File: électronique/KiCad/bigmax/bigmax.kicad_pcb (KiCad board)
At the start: 2 copper layers, 99.1 x 99.1 mm, 25 parts, among them SW1 SW_Push, U1 qtr-1rc_a, U10 batt_connector, U11 micro_start, U2 qtr-1rc_b, U3 dc_geared_encoder, U4 dc_geared_encoder, U5 TPS61090_dc_boost, U6 MT3608, U7 VL53L0X_a, U8 VL53L0X_b, U9 dc_driver_1A_3-14V

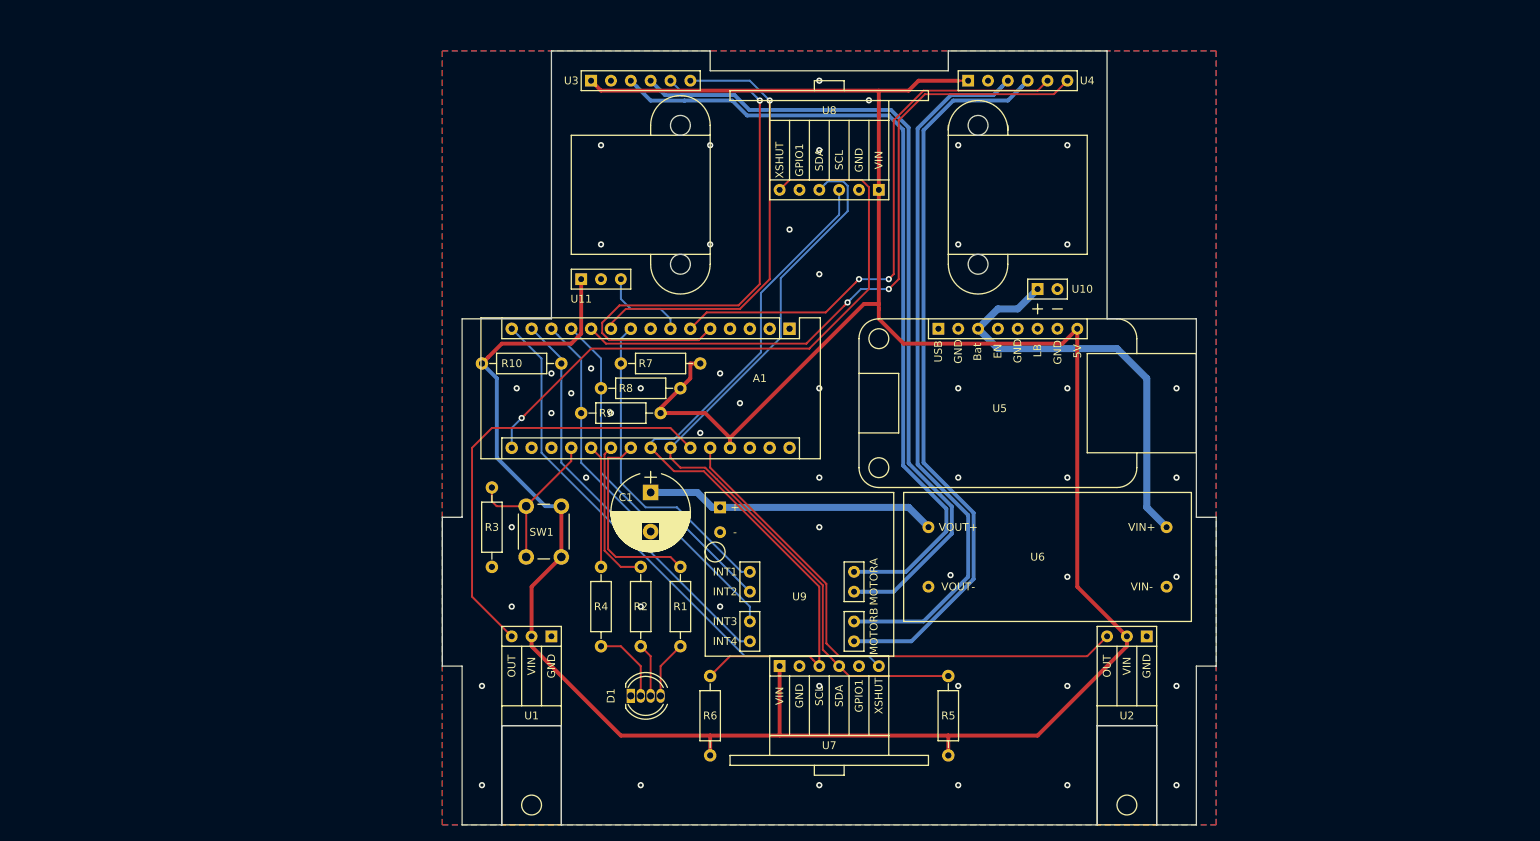
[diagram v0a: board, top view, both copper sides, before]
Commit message: Bigmax v2 - mai 2019
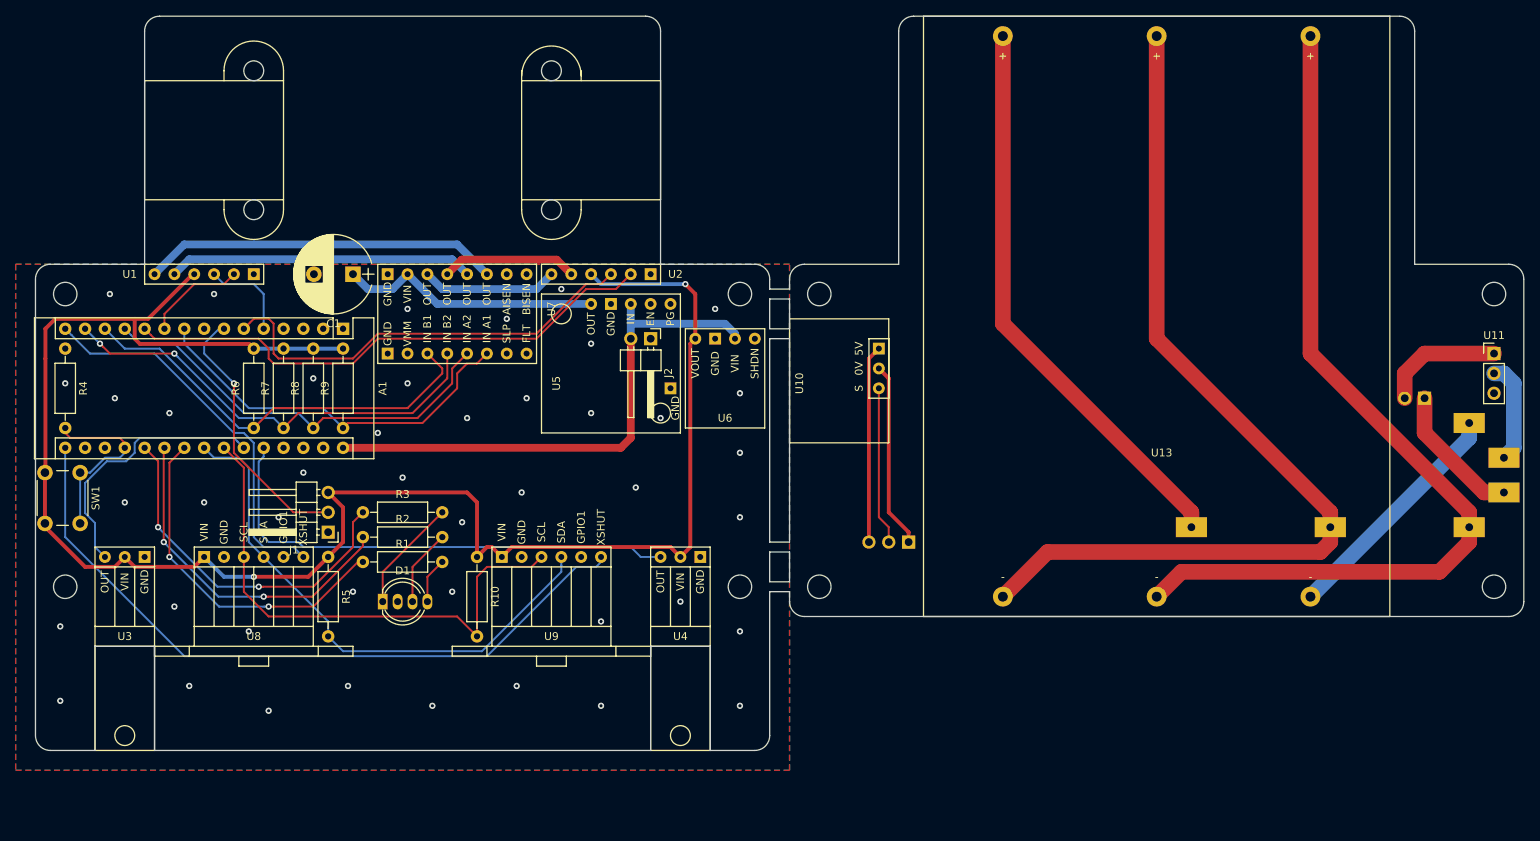
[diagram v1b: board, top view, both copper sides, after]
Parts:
- added J1: Conn_01x03, Pin_Headers:Pin_Header_Angled_1x03_Pitch2.54mm, F.Cu at (85.7, 112.4)
- added J2: Conn_01x02, Pin_Headers:Pin_Header_Angled_1x02_Pitch2.54mm, F.Cu at (127.0, 87.6)
- added J3: Conn_01x03_input, Pin_Headers:Pin_Header_Angled_1x03_Pitch2.54mm, B.Cu at (160.0, 113.7)
- added J4: Conn_01x02, Pin_Headers:Pin_Header_Angled_1x02_Pitch2.54mm, B.Cu at (226.1, 95.2)
- added U12: generic_bms_3s_10A, bigmax:generic_bms_3s_10A, B.Cu at (236.2, 102.9)
- added U13: generic_18650_3s_case, bigmax:CB-18650-PC6, F.Cu at (172.1, 48.9)
- D1: footprint LEDs:LED_D5.0mm-4 -> bigmax:LED_D5.0mm-4
- R3: value 1k -> 220
- R4: value 220 -> 1k
- U1: value qtr-1rc_a -> pololu_enc03b; footprint bigmax:qtr_1rc -> bigmax:pololu_enc03b
- U10: value batt_connector -> jsumo_micro_start; footprint bigmax:batt_connector -> bigmax:jsumo_micro_start
- U11: value micro_start -> generic_vertical_slide_switch; footprint bigmax:micro_start -> Pin_Headers:Pin_Header_Straight_1x03_Pitch2.54mm
- U2: value qtr-1rc_b -> pololu_enc03b; footprint bigmax:qtr_1rc -> bigmax:pololu_enc03b
- U3, U4: value dc_geared_encoder -> pololu_irs01a; footprint bigmax:dc_geared_encoder -> bigmax:pololu_irs01a
- U5: value TPS61090_dc_boost -> pololu_reg19a; footprint bigmax:dc_boost_500C -> bigmax:pololu_reg19a
- U6: value MT3608 -> pololu_reg04b; footprint bigmax:MT3608 -> bigmax:pololu_reg04b
- U7: value VL53L0X_a -> pololu_md17a; footprint bigmax:vl53l0x -> bigmax:pololu_md17a
- U8: value VL53L0X_b -> generic_vl53l0x; footprint bigmax:vl53l0x -> bigmax:generic_vl53l0x
- U9: value dc_driver_1A_3-14V -> generic_vl53l0x; footprint bigmax:MX1616 -> bigmax:generic_vl53l0x
- moved U11 117.2 mm to (234.9, 89.5)
- moved U8 98.3 mm to (69.8, 115.6), turned to 0 degrees
- moved U3 83.6 mm to (62.2, 115.6), turned to 180 degrees
- moved R5 80.8 mm to (85.7, 115.6)
- moved U2 78.6 mm to (127.0, 79.4)
- moved R4 74.1 mm to (52.1, 88.9)
- moved U4 69.9 mm to (133.3, 115.6), turned to 180 degrees
- moved R6 66.5 mm to (76.2, 99.1), turned to 90 degrees
- moved U7 64.2 mm to (93.3, 89.5), turned to 90 degrees
- moved U6 62.6 mm to (135.3, 87.6)
- moved SW1 61.7 mm to (54.0, 104.8)
- moved U1 60.0 mm to (76.2, 79.4)
- moved A1 57.2 mm to (87.6, 86.4)
- moved C1 47.2 mm to (88.9, 79.4), turned to 180 degrees
- moved R7 44.0 mm to (80.0, 99.1), turned to 90 degrees
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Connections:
- net Net-(A1-Pad21) renamed /led_green
- net Net-(A1-Pad22) renamed /led_blue
- A1 pad 1: Net-(A1-Pad1) -> (no net)
- A1 pad 17: Net-(A1-Pad17) -> (no net)
- A1 pad 18: Net-(A1-Pad18) -> (no net)
- A1 pad 2: Net-(A1-Pad2) -> (no net)
- A1 pad 20: Net-(A1-Pad20) -> /led_red
- A1 pad 27: VCC -> (no net)
- A1 pad 28: Net-(A1-Pad28) -> (no net)
- A1 pad 3: Net-(A1-Pad3) -> (no net)
- A1 pad 30: Net-(A1-Pad30) -> +12V
- A1 pad 8: Net-(A1-Pad8) -> (no net)
- D1 pad 1: GND -> Net-(D1-Pad1)
- D1 pad 2: Net-(D1-Pad2) -> GND
- R10 pad 1: /in4 -> +5V
- R10 pad 2: VCC -> /scl
- R3 pad 1: GND -> /led_red
- R3 pad 2: Net-(A1-Pad19) -> Net-(D1-Pad1)
- R4 pad 1: Net-(A1-Pad20) -> GND
- R4 pad 2: Net-(D1-Pad2) -> Net-(A1-Pad19)
- R5 pad 1: /scl -> +5V
- R5 pad 2: VCC -> /sda
- R6 pad 1: /sda -> /in3
- R6 pad 2: VCC -> +5V
- R7 pad 1: /in1 -> /in4
- R7 pad 2: VCC -> +5V
- R8 pad 2: VCC -> +5V
- R9 pad 1: /in3 -> /in1
- R9 pad 2: VCC -> +5V
- SW1 pad 1: VCC -> Net-(A1-Pad19)
- SW1 pad 2: Net-(A1-Pad19) -> +5V
- U1 pad 2: VCC -> /c2_a
- U1 pad 3: /out_a -> /c1_a
- U10 pad 1: +BATT -> Net-(J3-Pad3)
- U10 pad 2: GND -> Net-(J3-Pad1)
- U11 pad 1: VCC -> Net-(J4-Pad2)
- U11 pad 2: GND -> Net-(U11-Pad2)
- U11 pad 3: Net-(A1-Pad7) -> (no net)
- U2 pad 2: VCC -> /c2_b
- U2 pad 3: /out_b -> /c1_b
- U3 pad 1: VCC -> GND
- U3 pad 2: GND -> +5V
- U3 pad 3: /M1 -> /out_a
- U4 pad 1: VCC -> GND
- U4 pad 2: GND -> +5V
- U4 pad 3: /M3 -> /out_b
- U5 pad 1: Net-(U5-Pad1) -> (no net)
- U5 pad 2: GND -> (no net)
- U5 pad 3: +BATT -> +12V
- U5 pad 4: Net-(U5-Pad4) -> GND
- U5 pad 5: GND -> +6V
- U5 pad 6: Net-(U5-Pad6) -> GND
- U6 pad 1: +BATT -> +5V
- U6 pad 3: +6V -> +12V
- U6 pad 4: GND -> (no net)
- U7 pad 1: VCC -> GND
- U7 pad 2: GND -> (no net)
- U7 pad 3: /sda -> /in3
- U7 pad 4: /scl -> /in4
- U7 pad 5: Net-(U7-Pad5) -> /in2
- U7 pad 6: /XSHUT_a -> /in1
- U8 pad 1: VCC -> +5V
- U8 pad 3: /sda -> /scl
- U8 pad 4: /scl -> /sda
- U8 pad 5: Net-(U8-Pad5) -> (no net)
- U8 pad 6: /XSHUT_b -> /XSHUT_a
- U9 pad 1: +6V -> +5V
- U9 pad 3: /in1 -> /scl
- U9 pad 4: /in2 -> /sda
- U9 pad 5: /in3 -> (no net)
- U9 pad 6: /in4 -> /XSHUT_b
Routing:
- net VCC: track 360.2 -> 0.00 mm
- net +5V: track 0.00 -> 232.4 mm, vias 0 -> 2
- net /b2: track 0.00 -> 118.8 mm
- net /b1: track 0.00 -> 116.1 mm
- net /M4: track 94.7 -> 17.4 mm
- net /M3: track 91.1 -> 17.5 mm
- net /b+: track 0.00 -> 72.9 mm
- net +12V: track 0.00 -> 69.0 mm
- net /M2: track 105.4 -> 39.0 mm
- net /c1_a: track 74.3 -> 12.5 mm, vias 1 -> 0
- net /M1: track 105.1 -> 45.7 mm
- net +BATT: track 54.0 -> 0.00 mm
- net /led_red: track 0.00 -> 46.0 mm, vias 0 -> 2
- net /c2_a: track 57.4 -> 13.5 mm, vias 1 -> 0
- net /scl: track 100.5 -> 68.6 mm
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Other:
- board size 99.1 x 99.1 mm -> 190.5 x 94 mm
- board text added: "bigmax - v2.0.0 mai 2019"
- board text removed: "bigmax - v1.0.0 janvier 2019"
